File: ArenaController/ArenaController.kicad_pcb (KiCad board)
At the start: 2 copper layers, 86.6 x 104.5 mm, 45 parts, among them J1 RJ45, J2 RJ45, J3 5Pin_5mm_plus_2.54_pin, J4 RJ45, J5 RJ45, J6 RJ45, J7 Barrel_Jack, Q1 IRLIZ44N, Q2 IRLIZ44N, Q3 IRLIZ44N, Q4 IRLIZ44N, Q5 IRLIZ44N, U1 ESP32-DEVKIT-V1, U2 20mmx50mm_buckboost

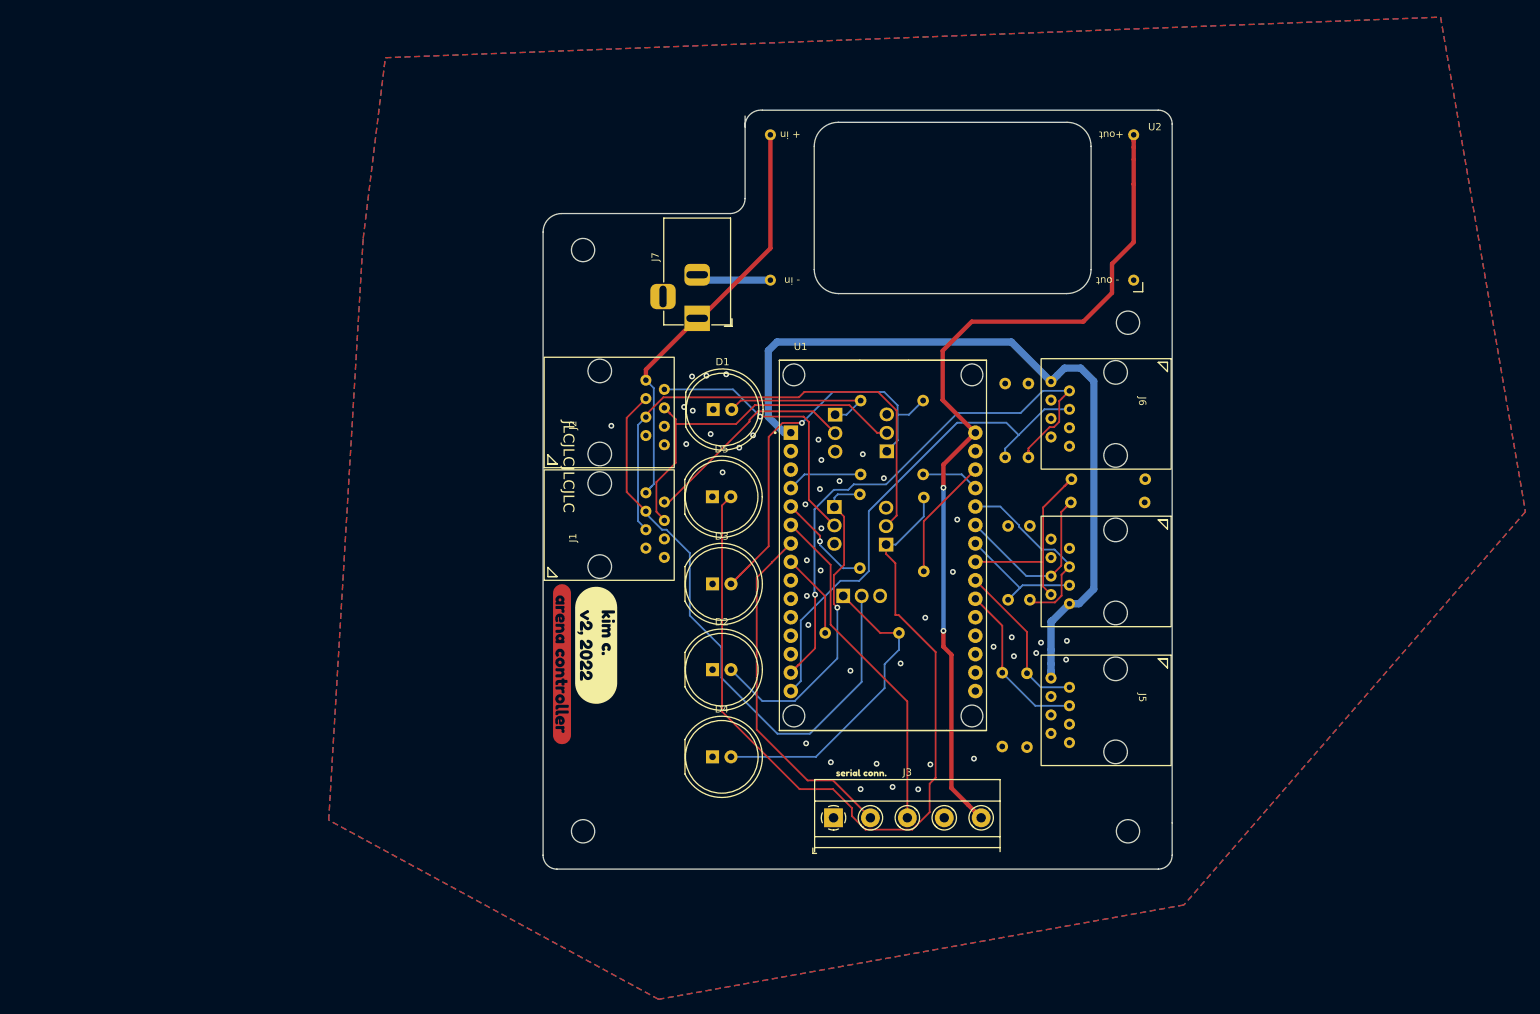
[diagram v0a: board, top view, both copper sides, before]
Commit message: Update to shit.
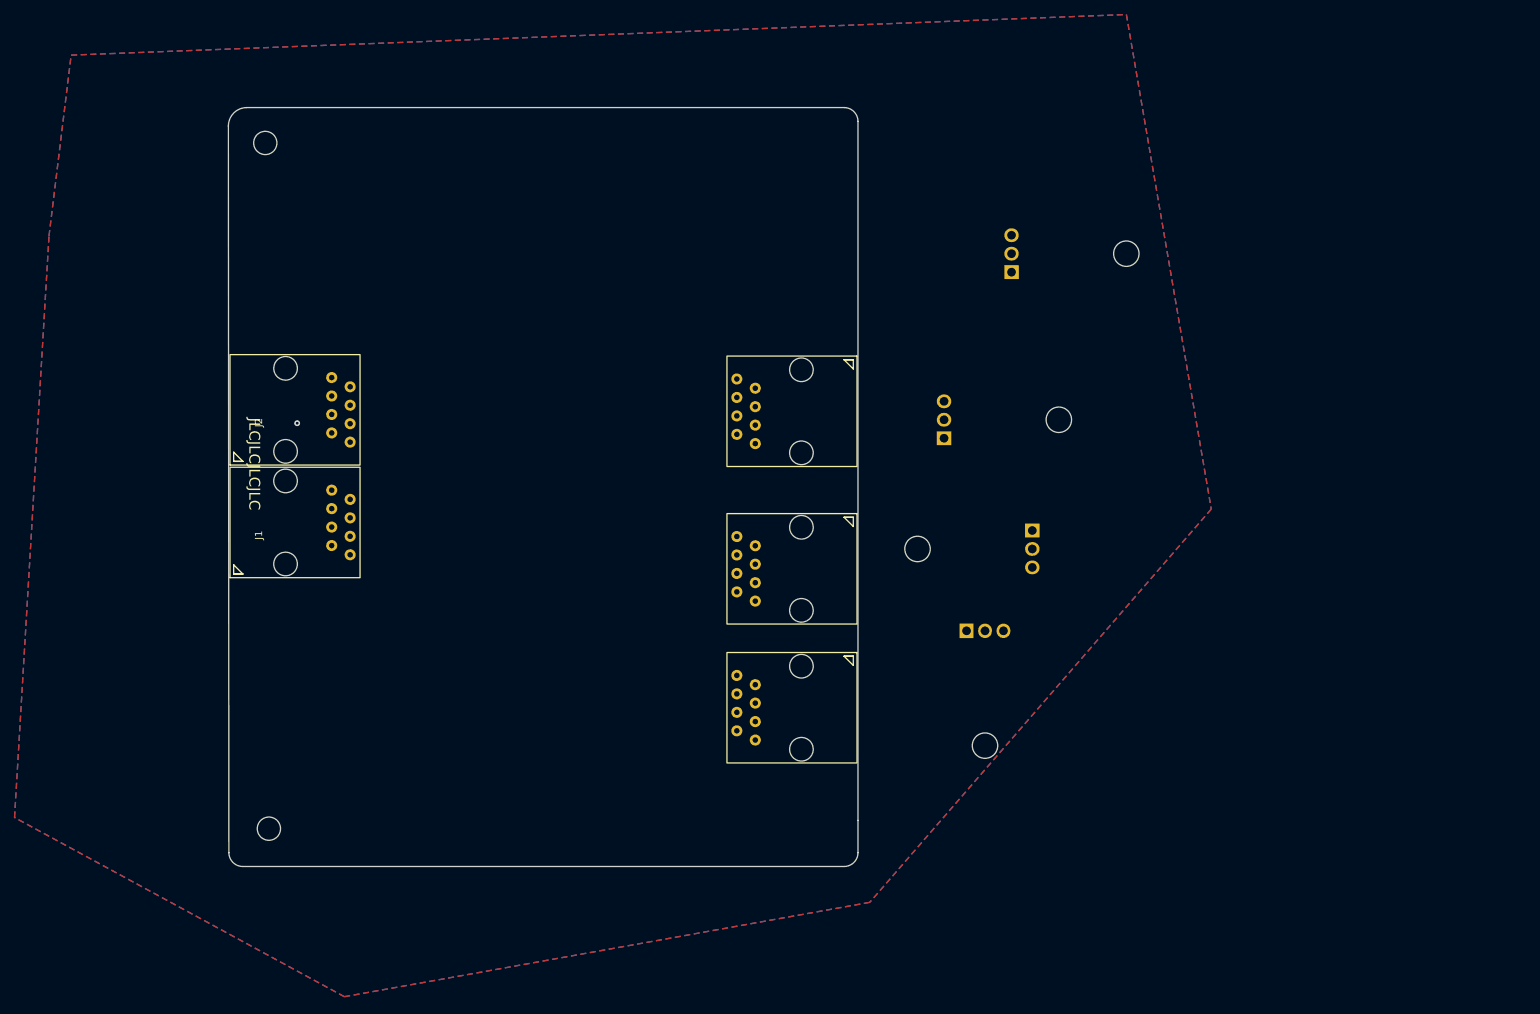
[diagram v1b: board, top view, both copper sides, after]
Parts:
- removed D1, D2: rLED, LED_THT:LED_D10.0mm
- removed D3: gLED, LED_THT:LED_D10.0mm
- removed D4: yLED, LED_THT:LED_D10.0mm
- removed D5: LED, LED_THT:LED_D10.0mm
- removed H3, H4: MountingHole, MountingHole:MountingHole_3.2mm_M3
- removed J3: 5Pin_5mm_plus_2.54_pin, footprints:5pin_5mmpitch_plus_2.54_combo
- removed J7: Barrel_Jack, Connector_BarrelJack:BarrelJack_Horizontal
- removed Q5: IRLIZ44N, Package_TO_SOT_THT:TO-220F-3_Vertical
- removed R1, R10, R11, R12, R13, R7, R8, R9: 10k, Resistor_THT:R_Axial_DIN0207_L6.3mm_D2.5mm_P10.16mm_Horizontal
- removed R2, R3, R4, R5, R6: 330, Resistor_THT:R_Axial_DIN0207_L6.3mm_D2.5mm_P10.16mm_Horizontal
- removed U1: ESP32-DEVKIT-V1, ESP32DK1:MODULE_ESP32_DEVKIT_V1
- removed U2: 20mmx50mm_buckboost, footprints:buckboost_mount
- removed kibuzzard-63898CDD: G***, kibuzzard-63898CDD
- removed kibuzzard-638A2249, kibuzzard-638A2249123: G***, kibuzzard-638A2249
- removed kibuzzard-638A2274: G***, kibuzzard-638A2274
- Q1, Q2, Q3, Q4: footprint Package_TO_SOT_THT:TO-220F-3_Vertical -> Package_TO_SOT_THT:TO-220F-3_Horizontal_TabDown
- moved H1 46.2 mm to (48.3, 48.3)
- moved J4 43.2 mm to (129.7, 99.3)
- moved J5 43.2 mm to (129.7, 118.4)
- moved J6 43.2 mm to (129.7, 77.6)
- moved kibuzzard-638A2165 43.2 mm to (128.3, 126.5)
- moved kibuzzard-638A2178 43.2 mm to (128.1, 85.1)
- moved H2 43.2 mm to (48.8, 142.6)
- moved J1 43.2 mm to (43.4, 108.1)
- moved J2 43.2 mm to (43.4, 92.6)
- moved kibuzzard-638A2138 43.2 mm to (46.7, 85.1)
- moved kibuzzard-638A214B 43.2 mm to (46.7, 100.5)
- moved kibuzzard-638A219C 43.2 mm to (126.9, 106.9)
- moved Q2 31.5 mm to (153.8, 101.6)
- moved Q1 30.0 mm to (151.0, 66.0)
- moved Q4 17.6 mm to (144.8, 115.4)
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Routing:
- net +5V: track 132.6 -> 0.00 mm, vias 2 -> 0
- net Net-(D5-A): track 116.7 -> 0.00 mm
- net +3V3: track 110.0 -> 0.00 mm
- net /s_Yellow: track 82.2 -> 0.00 mm
- net /T_A_End: track 78.4 -> 0.00 mm, vias 1 -> 0
- net /s_Horn: track 69.7 -> 0.00 mm
- net /T_A_Start: track 68.3 -> 0.00 mm
- net +12V: track 64.7 -> 0.00 mm
- net Net-(D3-A): track 58.4 -> 0.00 mm, vias 1 -> 0
- net /s_Green: track 50.4 -> 0.00 mm
- net /Dis_Serial_Tx: track 48.2 -> 0.00 mm
- net /Dis_serial_Rx: track 46.9 -> 0.00 mm
- net Net-(D2-Pad2): track 46.0 -> 0.00 mm, vias 1 -> 0
- net Net-(D4-A): track 43.3 -> 0.00 mm
- net /s_Red_2: track 37.4 -> 0.00 mm, vias 1 -> 0
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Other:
- board size 86.6 x 104.5 mm -> 86.7 x 104.5 mm
